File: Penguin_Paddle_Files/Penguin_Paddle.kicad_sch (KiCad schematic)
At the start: 15 parts, among them J1 Conn_01x01_Socket, J2 AudioPlug3, J3 Conn_01x01_Socket, Q1 NPN, SW1 SW_SPST, SW2 SW_SPST, U1 XIAO-ESP32-S3-DIP

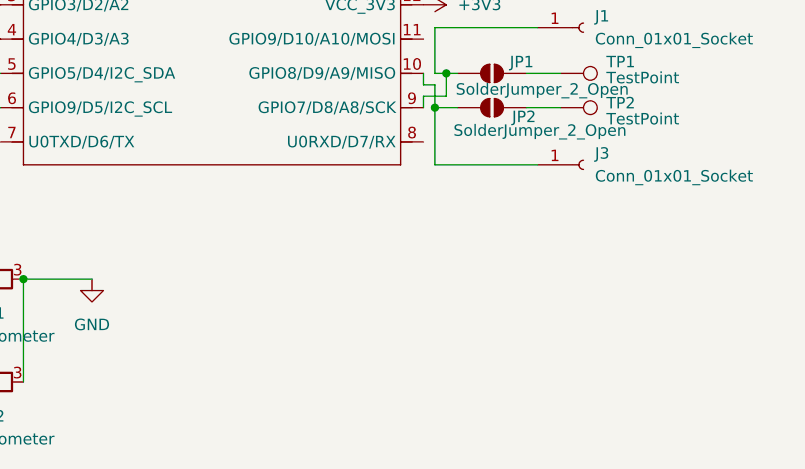
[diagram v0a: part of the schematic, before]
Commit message: Cleaned folders (frogot to commit this a few days ago)
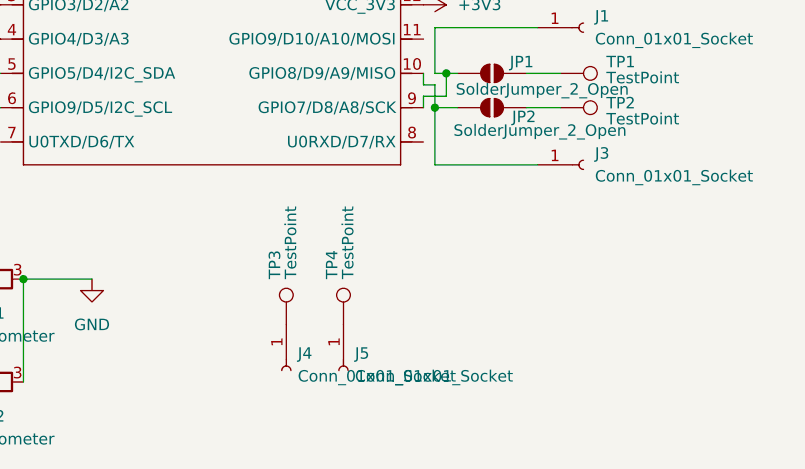
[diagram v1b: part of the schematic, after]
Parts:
- added J4, J5: Conn_01x01_Socket, Connector_Wire:SolderWire-0.1sqmm_1x01_D0.4mm_OD1mm, symbol Connector:Conn_01x01_Socket
- added TP3, TP4: TestPoint, Custom:Copper Pad, symbol Connector:TestPoint
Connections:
- new net: J5.1 (Pin_1), TP4.1
- new net: J4.1 (Pin_1), TP3.1
